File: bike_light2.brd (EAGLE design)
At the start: 22.1 x 22.1 mm, 6 parts

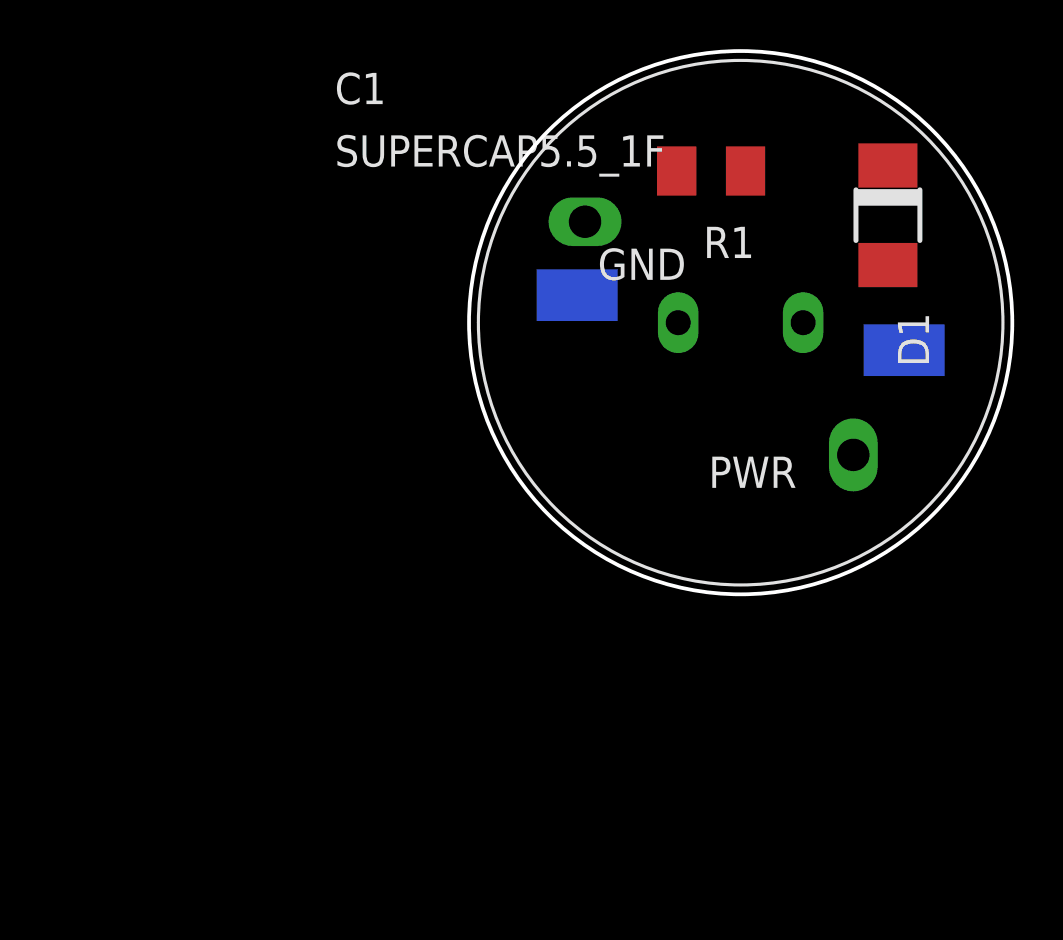
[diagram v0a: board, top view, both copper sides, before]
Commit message: Latest light after the first build.
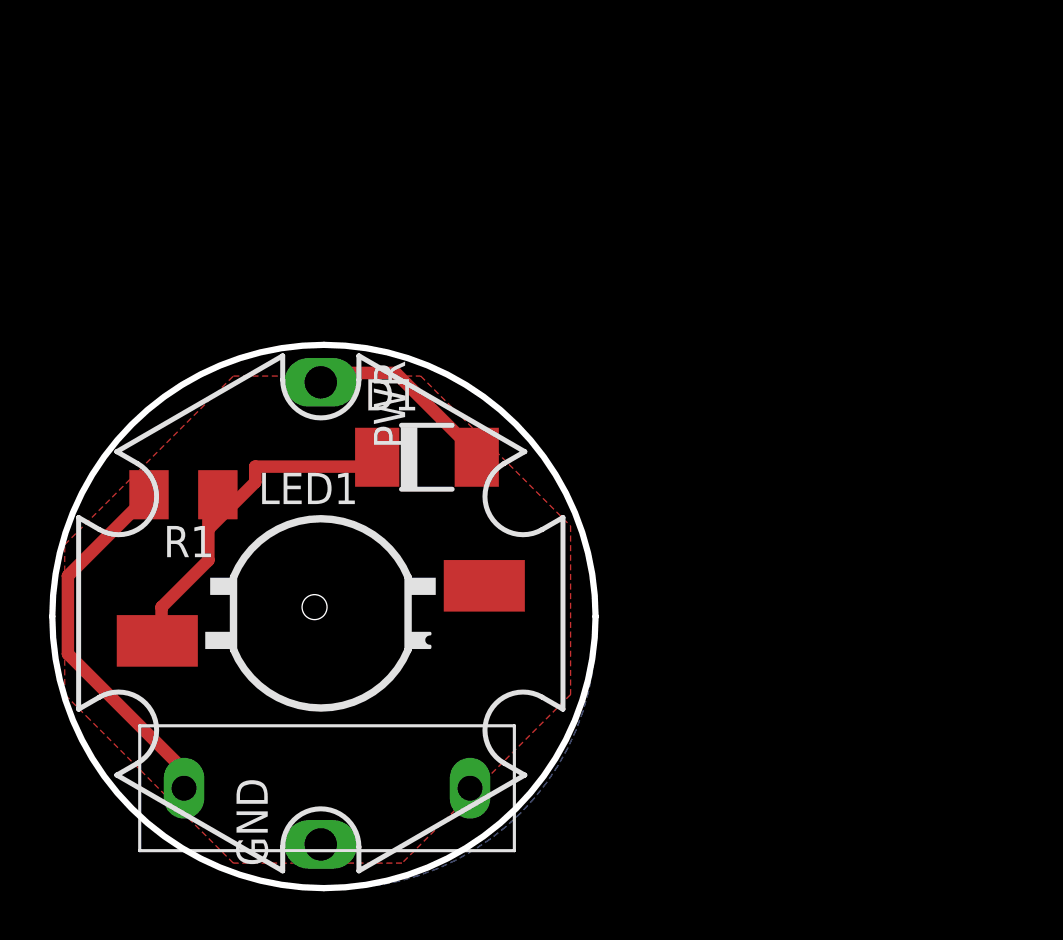
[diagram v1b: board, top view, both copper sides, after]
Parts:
- C1: value SUPERCAP5.5_1F -> SUPERCAP5.5_1FDGH; device christy:SUPERCAP5.5_1F -> christy:CAP_1UF_DGH
- moved GND 27.5 mm to (10.9, 1.78)
- moved C1 25.3 mm to (11.2, 4.06)
- moved R1 25.2 mm to (5.33, 16.0)
- moved PWR 21.9 mm to (10.9, 20.6), turned to 270 degrees
- moved D1 21.2 mm to (15.2, 17.5), turned to 0 degrees
- moved LED1 20.8 mm to (10.9, 11.2), flipped to the top
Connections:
- net N$3 renamed GND
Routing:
- net N$1: track 0.00 -> 15.5 mm
- net N$5: track 0.00 -> 15.2 mm
- net N$4: track 0.00 -> 7.95 mm
- added copper zone on layer 1, net GND
- added copper zone on layer 16, net GND
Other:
- outline, holes or cut-outs redrawn
